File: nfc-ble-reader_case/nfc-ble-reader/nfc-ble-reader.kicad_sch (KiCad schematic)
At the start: 6 parts, among them SW1 SW_DPST_x2, U1 nRF52840_ProMicro_NiceNano, U2 PN532_NFC_Elechouse_HW147_SPI

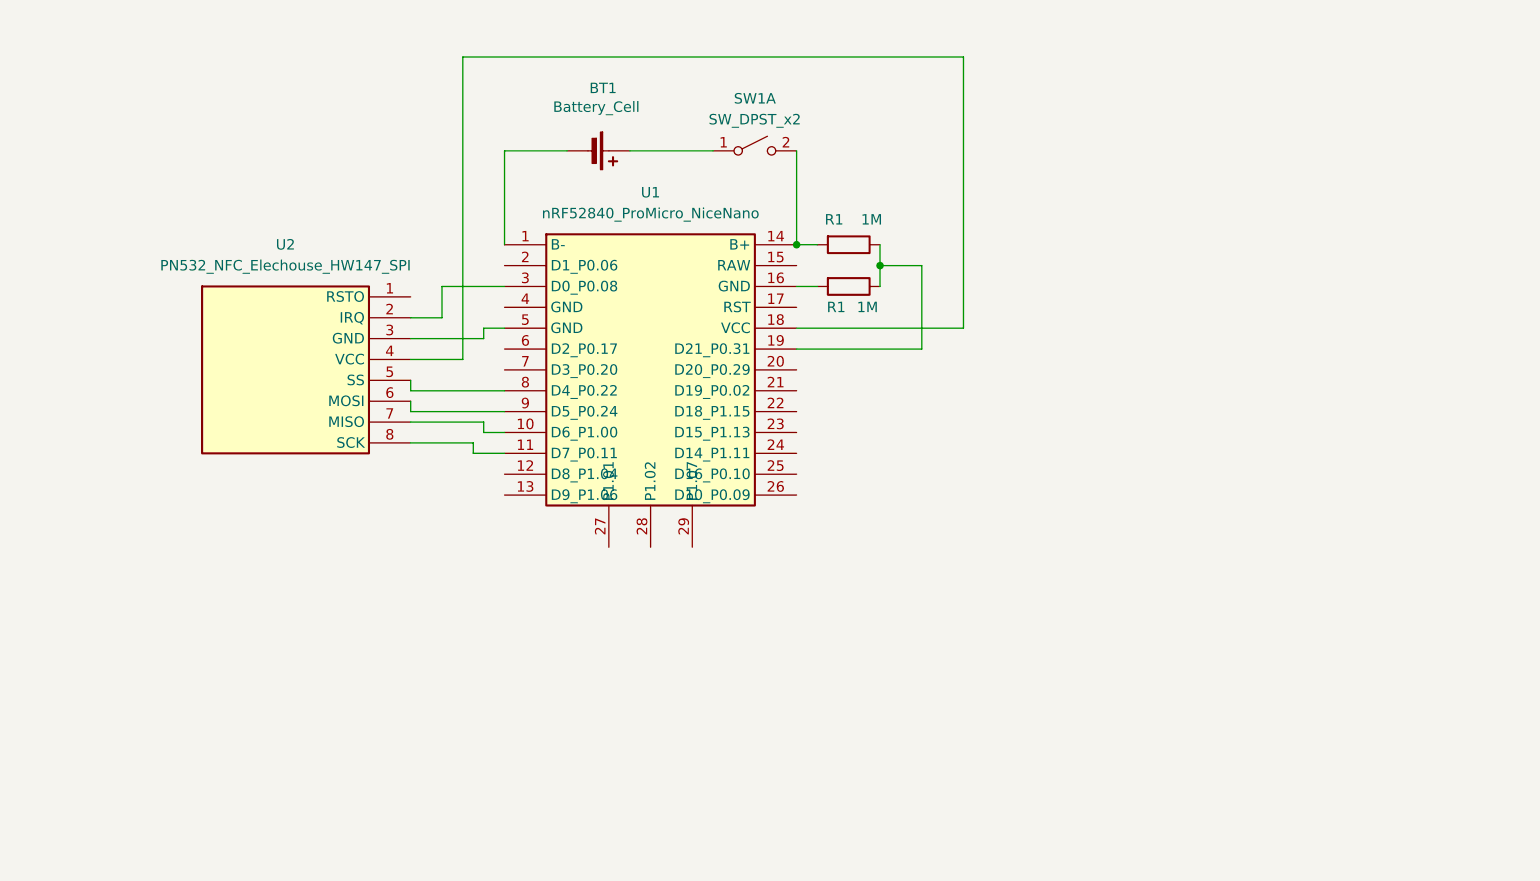
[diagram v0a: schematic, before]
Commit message: KiCad PCB with Components New LOGO Images for different layouts
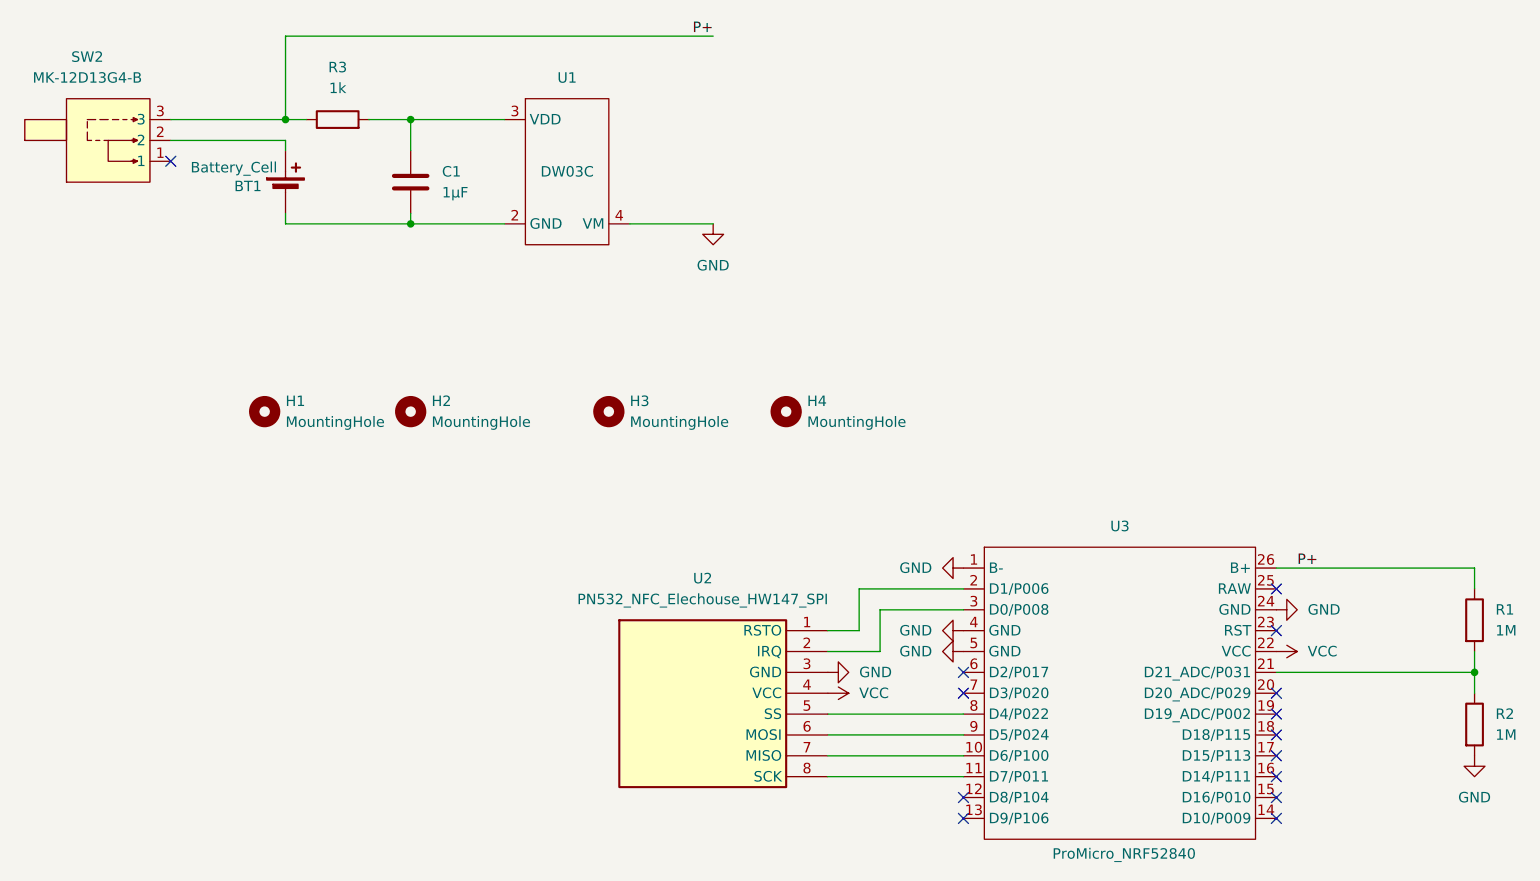
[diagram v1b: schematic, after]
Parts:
- removed R1 (x2): 1M, symbol Device:R
- removed SW1: SW_DPST_x2, symbol Switch:SW_DPST_x2
- removed U1: nRF52840_ProMicro_NiceNano, symbol symbols:nRF52840_ProMicro_NiceNano
- added C1: 1µF, Capacitor_SMD:C_0805_2012Metric_Pad1.18x1.45mm_HandSolder, symbol Device:C
- added H1, H2: MountingHole, MountingHole:MountingHole_3.2mm_M3, symbol Mechanical:MountingHole
- added H3, H4: MountingHole, MountingHole:MountingHole_6.4mm_M6, symbol Mechanical:MountingHole
- added R1, R2: 1M, Resistor_SMD:R_0805_2012Metric_Pad1.20x1.40mm_HandSolder, symbol Device:R
- added R3: 1k, Resistor_SMD:R_0805_2012Metric_Pad1.20x1.40mm_HandSolder, symbol Device:R
- added SW2: MK-12D13G4-B, HOOYA_MK-12D13G4-B:SW-TH_MK-12D13G4-B, symbol HOOYA_MK-12D13G4-B:MK-12D13G4-B
- added U1: DW03C, Package_TO_SOT_SMD:SOT-23-5_HandSoldering, symbol project:DW03C
- added U3: ProMicro_NRF52840, Library:ProMicro_NRF52840, symbol project:proMicro_nrf52840
- BT1: footprint (none) -> 18650_Battery_Holder_SMD:BATTERY-SMD_18650-1S-L77.1-W20.7-1
- U2: footprint (none) -> Connector_PinSocket_2.54mm:PinSocket_1x08_P2.54mm_Vertical
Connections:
- net at BT1.1 (+): now also SW2.2
- net at BT1.2 (-): now also C1.2, U1.2 (GND)
- net at U2.7 (MISO): now also U3.10 (D6/P100)
- net at U2.8 (SCK): now also U3.11 (D7/P011)
- net VCC: now reaches U2.4 (VCC)
- net VCC: now also U3.22 (VCC)
- net at U2.2 (IRQ): now also U3.3 (D0/P008)
- net GND: now reaches U2.3 (GND)
- net GND: now also R2.2, U1.4 (VM), U3.1 (B-), U3.24 (GND), U3.4 (GND), U3.5 (GND)
- net at U2.5 (SS): now also U3.8 (D4/P022)
- net at U2.6 (MOSI): now also U3.9 (D5/P024)
- net at U2.1 (RSTO): now also U3.2 (D1/P006)
- new net: R1.2, R2.1, U3.21 (D21_ADC/P031)
- new net: C1.1, R3.2, U1.3 (VDD)
- new net P+: R1.1, R3.1, SW2.3, U3.26 (B+)
- no-connect marks 0 -> 14
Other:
- moved on the sheet: BT1, U2

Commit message: finalized first pcb design and ordered 10 PCBs and components for 20 devices and 100 batteries
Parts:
- BT1: LCSC Part (none) -> C2988620
- C1: LCSC Part (none) -> C46653
- R1, R2: LCSC Part (none) -> C2907302
- R3: LCSC Part (none) -> C2907232
- U1: LCSC Part (none) -> C42380663
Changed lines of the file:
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@@
+			)
+		)
+		(property "LCSC Part" "C2907302"
+			(at 195.58 104.14 0)
+			(hide yes)
+			(show_name no)
+			(do_not_autoplace no)
+			(effects
+				(font
+					(size 1.27 1.27)
+				)
 			)
 		)
@@
 			)
 		)
+		(property "LCSC Part" "C46653"
+			(at 66.04 38.1 0)
+			(hide yes)
+			(show_name no)
+			(do_not_autoplace no)
+			(effects
+				(font
+					(size 1.27 1.27)
+				)
+			)
+		)
 		(pin "2"
 		)
@@
 		)
 		(property "Sim.Pins" "1=+ 2=-"
+			(at 50.8 39.37 0)
+			(hide yes)
+			(show_name no)
+			(do_not_autoplace no)
+			(effects
+				(font
+					(size 1.27 1.27)
+				)
+			)
+		)
+		(property "LCSC Part" "C2988620"
 			(at 50.8 39.37 0)
 			(hide yes)
@@
 			)
 		)
+		(property "LCSC Part" "C42380663"
+			(at 85.09 36.83 0)
+			(hide yes)
+			(show_name no)
+			(do_not_autoplace no)
+			(effects
+				(font
+					(size 1.27 1.27)
+				)
+			)
+		)
 		(pin "3"
 		)
@@
 			)
 		)
+		(property "LCSC Part" "C2907302"
+			(at 195.58 91.44 0)
+			(hide yes)
+			(show_name no)
+			(do_not_autoplace no)
+			(effects
+				(font
+					(size 1.27 1.27)
+				)
+			)
+		)
 		(pin "2"
 		)
@@
 			(hide yes)
 			(show_name no)
+			(do_not_autoplace no)
+			(effects
+				(font
+					(size 1.27 1.27)
+				)
+			)
+		)
+		(property "LCSC Part" "C2907232"
+			(at 57.15 30.48 90)
+			(hide yes)
+			(show_name no)
